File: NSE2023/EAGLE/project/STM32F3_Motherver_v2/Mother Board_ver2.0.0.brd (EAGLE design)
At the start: 50 x 35 mm, 36 parts, among them SW1 SRIDE_SWITCH

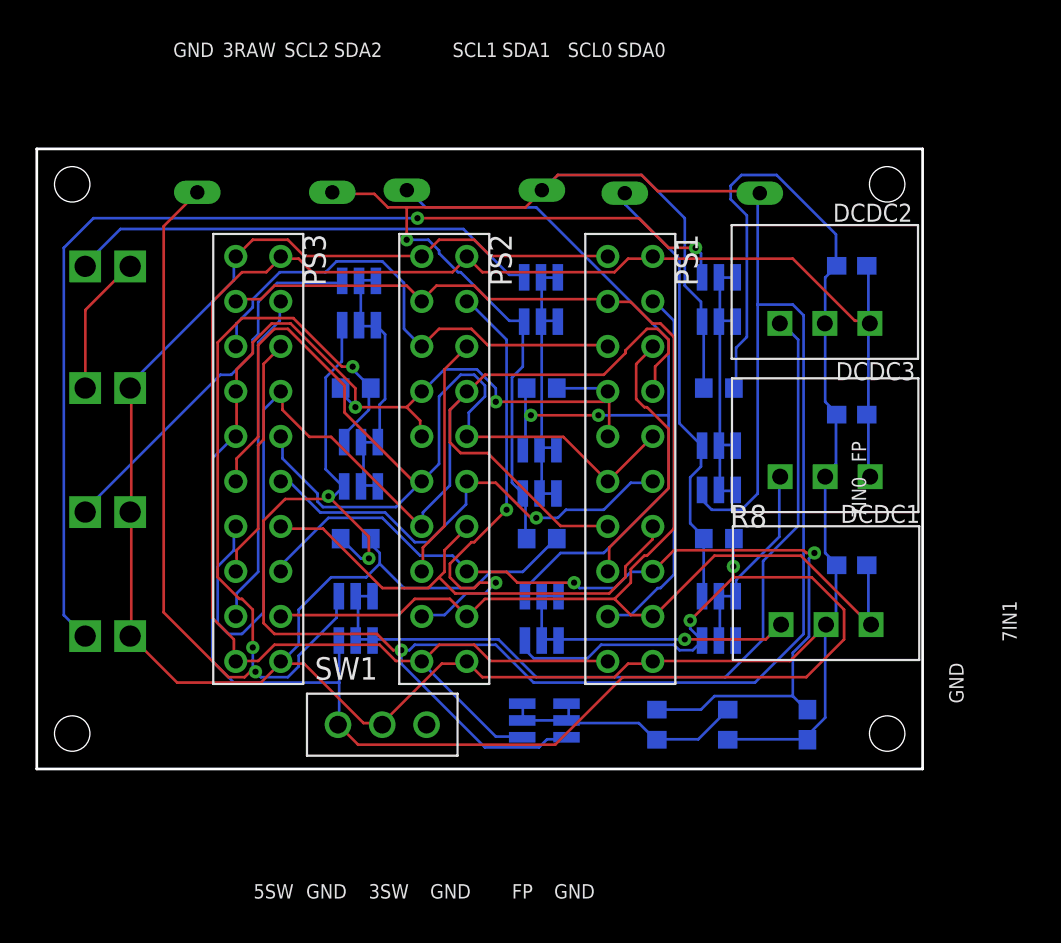
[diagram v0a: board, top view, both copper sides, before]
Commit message: www
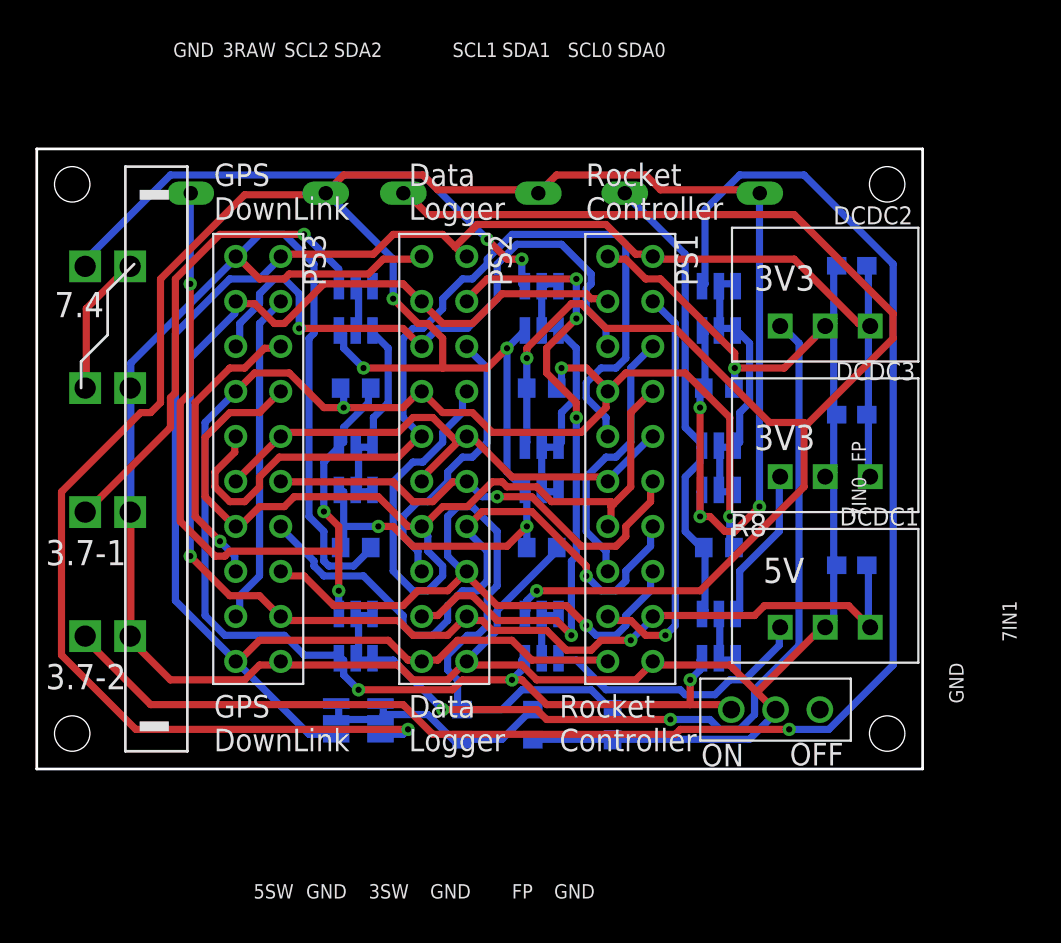
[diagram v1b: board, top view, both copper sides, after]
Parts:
- moved SW1 22.2 mm to (41.7, 3.35)
- moved C3 11.0 mm to (32.5, 2.50)
- moved R3 11.0 mm to (24.0, 2.50)
- moved R6 11.0 mm to (28.0, 2.50)
- moved MOS5 10.5 mm to (18.1, 2.74)
- moved MOS1 1.00 mm to (28.5, 7.50)
- moved MOS10 1.00 mm to (38.5, 7.50)
- moved MOS2 1.00 mm to (18.0, 7.50)
- moved MOS7 0.50 mm to (28.5, 26.0)
- moved MOS8 0.50 mm to (38.5, 26.0)
- moved R1 0.50 mm to (28.5, 12.5)
- moved R2 0.50 mm to (18.0, 12.5)
- moved R8 0.50 mm to (38.5, 12.5)
- moved D2 0.37 mm to (12.5, 32.5)
- moved MOS6 0.36 mm to (18.0, 17.0)
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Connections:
- net FPRAW: now also PS2.P$12, PS3.P$12
- net SW: no longer PS2.P$12, PS3.P$12
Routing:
- net FPRAW: track 0.00 -> 51.6 mm
- net N$11: track 49.2 -> 86.6 mm
- net N$1: track 73.3 -> 42.8 mm
- net 3.3_RAW4: track 61.3 -> 90.2 mm, vias 2 -> 1
- net SW: track 124.7 -> 97.3 mm, vias 4 -> 6
- net LOGTX: track 57.9 -> 31.9 mm
- net FP: track 183.9 -> 171.0 mm, vias 4 -> 9
- net SDA1: track 25.9 -> 38.2 mm, vias 2 -> 4
- net LOGRX: track 73.1 -> 63.3 mm
- net BIT2: track 28.9 -> 35.4 mm, vias 0 -> 1
- net PWM: track 28.3 -> 34.3 mm, vias 0 -> 1
- net 3.3_RAW3: track 21.5 -> 27.3 mm, vias 0 -> 1
- net N$5: track 47.4 -> 51.5 mm, vias 0 -> 2
- net 3.3_RAW1: track 26.9 -> 30.8 mm, vias 0 -> 2
- net +3V3: track 104.4 -> 108.0 mm
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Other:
- board text added: "-"
- board text added: "3.7-1"
- board text added: "3.7-2"
- board text added: "3V3"
- board text added: "5V"
- board text added: "7.4"
- board text added: "Data Logger"
- board text added: "GPS DownLink"
- board text added: "OFF"
- board text added: "ON"
- board text added: "Rocket Controller"
